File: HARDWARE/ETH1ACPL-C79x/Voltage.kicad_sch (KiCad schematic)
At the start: 60 parts, among them J501 1710072, U501 OPA340UA, U502 TBA 1-0511HI, U504 ACPL-C79B, U505 DG412LEDQ, U506 DG419LEDY, U507 DG412LEDQ, U509 OPA340UA, U510 OPA340UA

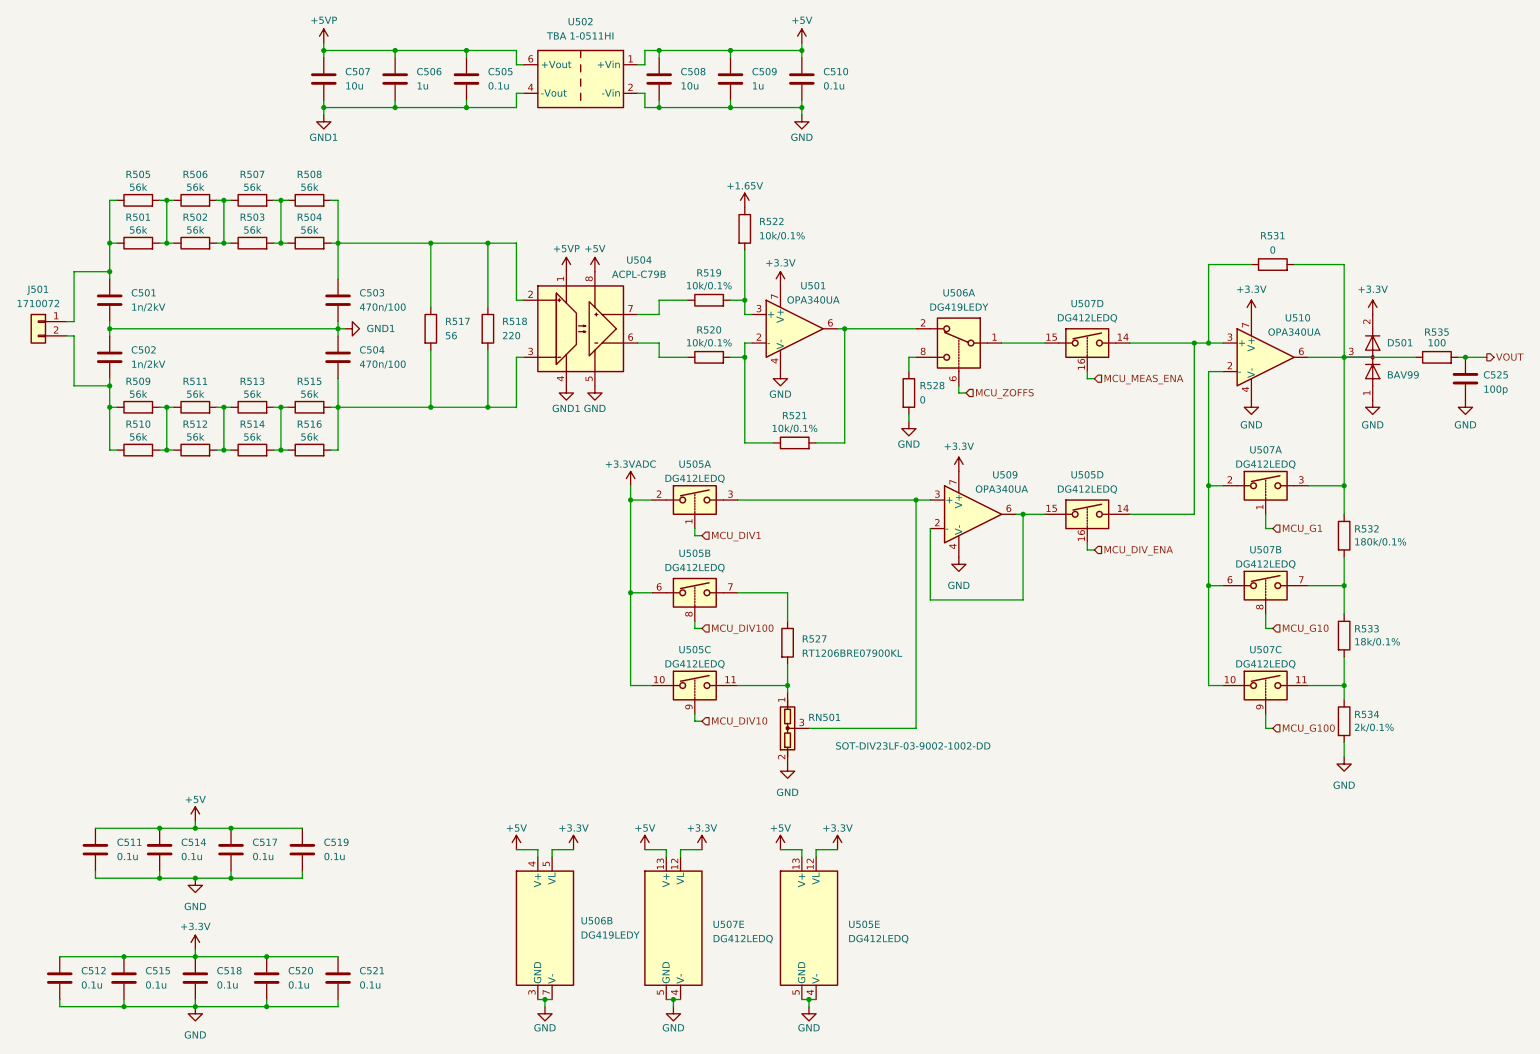
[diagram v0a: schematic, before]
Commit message: Development
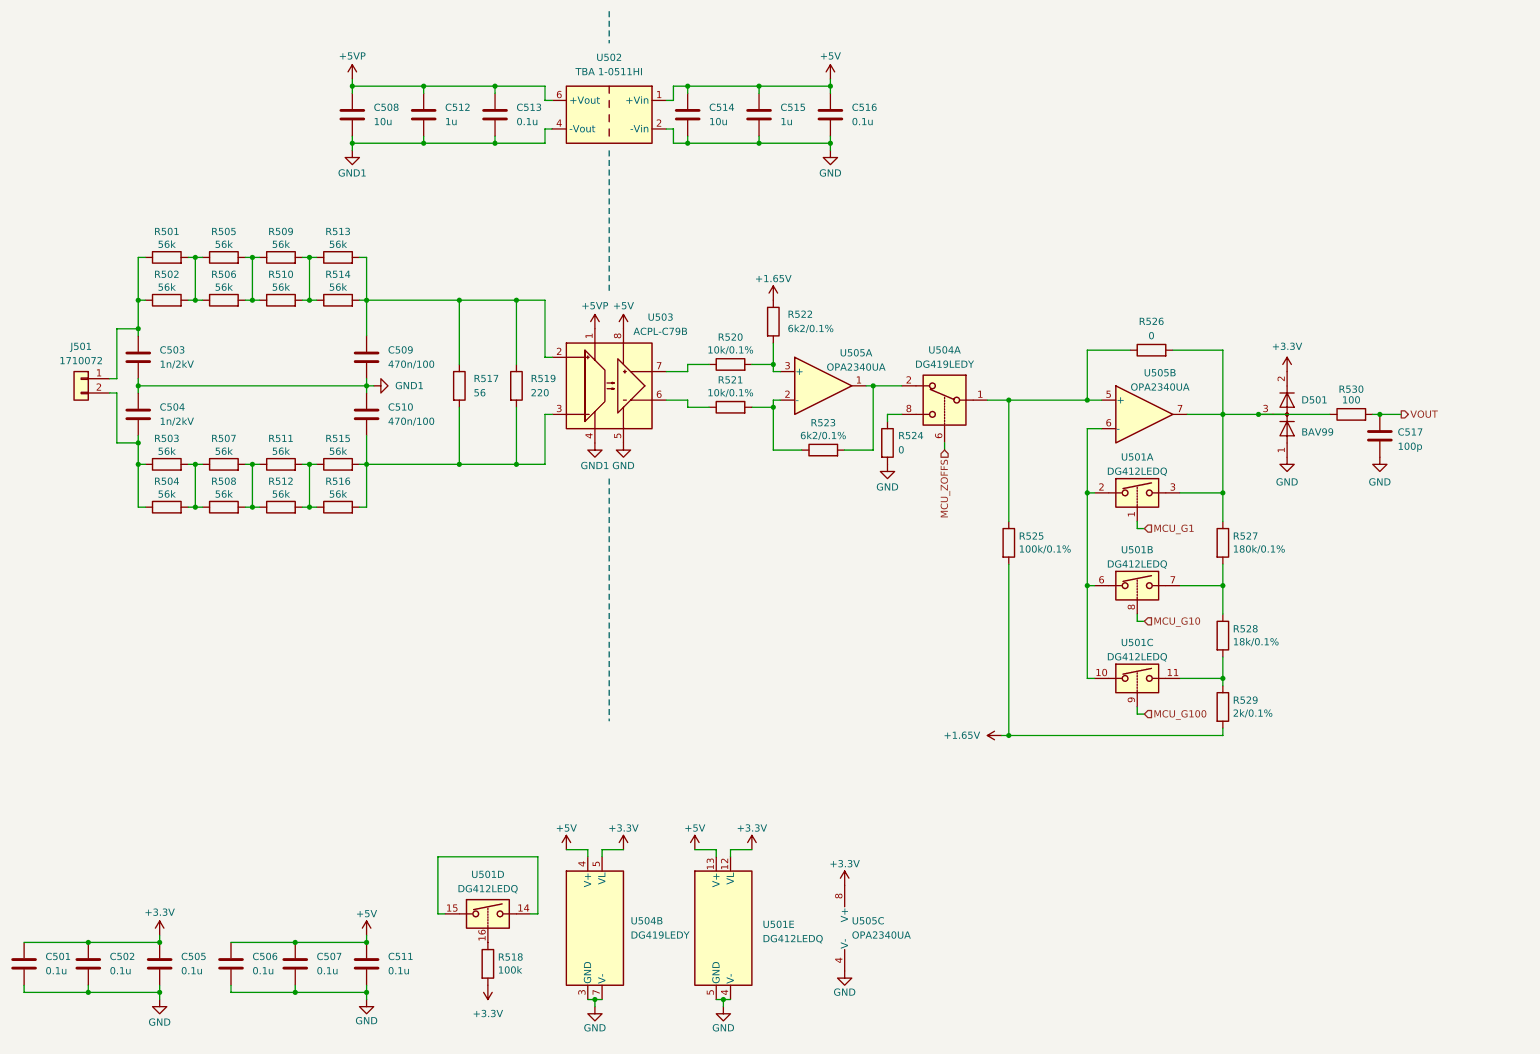
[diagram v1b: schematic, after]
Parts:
- removed C519, C520, C521: 0.1u, Capacitor_SMD:C_0603_1608Metric_Pad1.08x0.95mm_HandSolder, symbol Device:C
- removed R527: RT1206BRE07900KL, Resistor_SMD:R_1206_3216Metric_Pad1.30x1.75mm_HandSolder, symbol Device:R
- removed RN501: SOT-DIV23LF-03-9002-1002-DD, Package_TO_SOT_SMD:SOT-23, symbol Device:VoltageDivider_CenterPin3
- removed U501, U509, U510: OPA340UA, Package_SO:SOIC-8_3.9x4.9mm_P1.27mm, symbol Amplifier_Operational:OPA340UA
- removed U505: DG412LEDQ, Package_SO:TSSOP-16_4.4x5mm_P0.65mm, symbol Analog_Switch:DG412xUE
- added R518: 100k, Resistor_SMD:R_0603_1608Metric_Pad0.98x0.95mm_HandSolder, symbol Device:R
- added R525: 100k/0.1%, Resistor_SMD:R_0603_1608Metric_Pad0.98x0.95mm_HandSolder, symbol Device:R
- added U505: OPA2340UA, Package_SO:SOIC-8_3.9x4.9mm_P1.27mm, symbol Amplifier_Operational:OPA2340
- R522: value 10k/0.1% -> 6k2/0.1%
- R523: renamed from R521; value 10k/0.1% -> 6k2/0.1%
- U502: footprint (none) -> ETH1ACPL-C79x:TBA1
- renumbered C512 to C501, C515 to C502, C501 to C503, C502 to C504, C518 to C505, C511 to C506, C514 to C507, C507 to C508, C503 to C509, C504 to C510, C517 to C511, C506 to C512, C505 to C513, C508 to C514, C509 to C515, C510 to C516, C525 to C517, R505 to R501, R501 to R502, R509 to R503, R510 to R504, R506 to R505, R502 to R506, R511 to R507, R512 to R508, R507 to R509, R503 to R510, R513 to R511, R514 to R512, R508 to R513, R504 to R514, R518 to R519, R519 to R520, R520 to R521, R528 to R524, R531 to R526, R532 to R527, R533 to R528, R534 to R529, R535 to R530, U507 to U501, U504 to U503, U506 to U504
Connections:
- net +1.65V: now also R529.2, R525.2
- net +3.3V: now also R518.2, U505.8 (V+)
- net GND: now also U505.4 (V-); no longer R529.2
- net at R520.2, R522.2: now also U505.3 (+)
- net at D501.3 (K), R526.2, R527.1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: now also U505.7
- net at R521.2, R523.1: now also U505.2 (-)
- net at R523.2, U504.2: now also U505.1
- net at R526.1: now also U504.1, R525.1, U505.5 (+); no longer U501.14
- net at U501.15: now also U501.14; no longer U504.1
- net at U501.10, U501.2, U501.6: now also U505.6 (-)
- net MCU_MEAS_ENA: no longer names the net of U501.16
- net MCU_MEAS_ENA: now also R518.1
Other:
- moved on the sheet: C501, C502, C503, C504, C505, C506, C507, C508, C509, C510, C511, C512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
